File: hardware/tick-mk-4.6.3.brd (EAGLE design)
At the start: 96 x 53 mm, 40 parts, among them IC1 ATMEGA328P, IC2 DS3231, IC3 L7805, Y1 16MHz

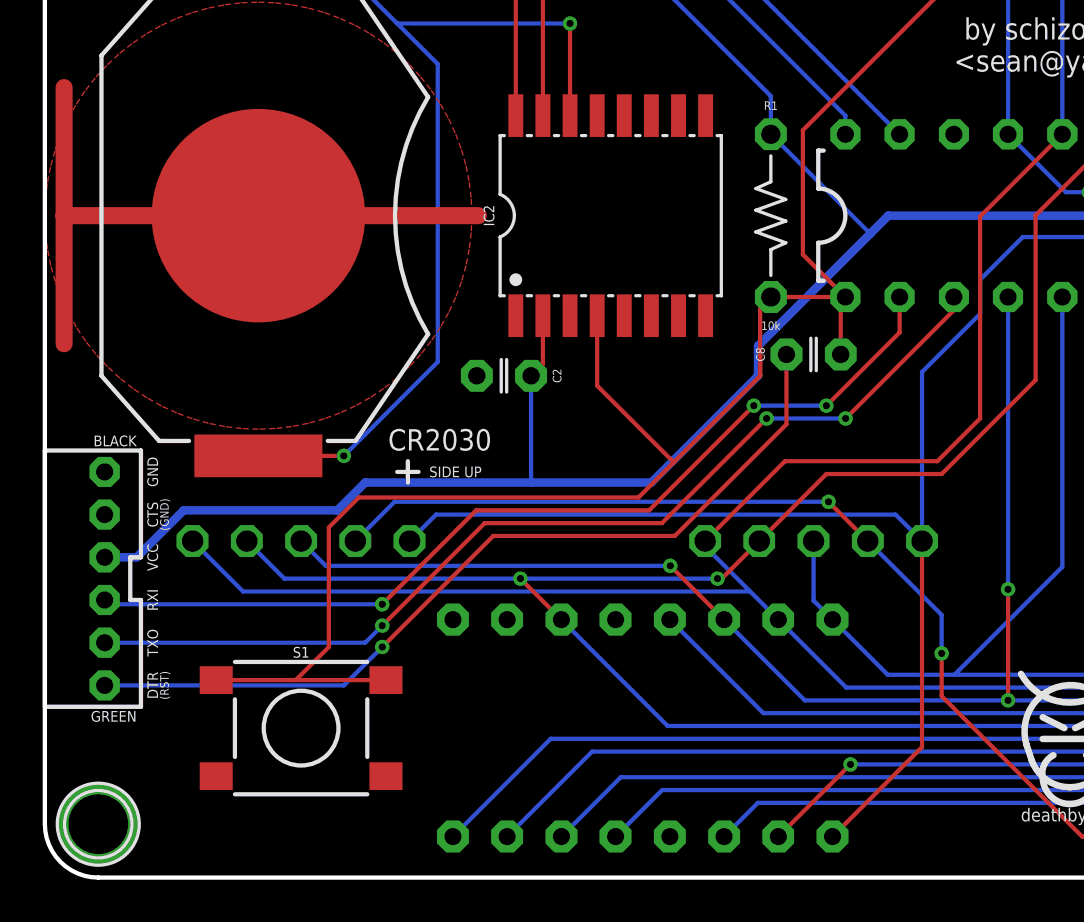
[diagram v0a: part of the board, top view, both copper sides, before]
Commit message: think i'm done fiddling
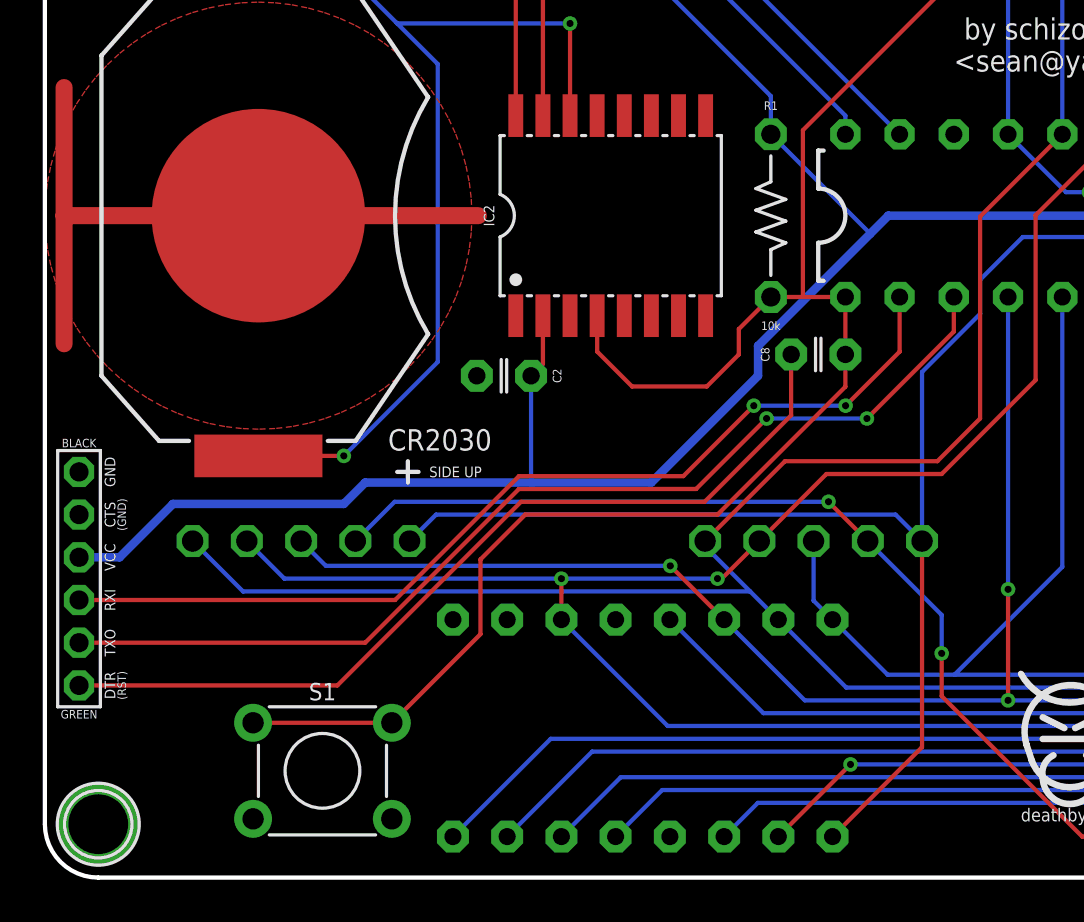
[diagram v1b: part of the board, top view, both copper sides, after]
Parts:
- JP1: value FTDI_CONNJST_PH_VERT_PTH -> FTDI_CONNJST_PH_VERT_PTH_LESSSILK; device A_butts:FTDI_CONN_JST_PH_VERT_PTH -> A_butts:FTDI_CONN_JST_PH_RA_PTH_LESSSILK
- S1: value SPST-NO-TACT6MM-SMD -> SPST-NO-TACT6MM-PTH-SMALL-PADS; device A_butts:DTSM-6 -> A_butts:DTS-6-SMALL-PADS
- moved S1 2.24 mm to (13.0, 5.00)
- moved JP1 1.20 mm to (1.60, 14.0)
- moved C8 0.22 mm to (36.2, 24.5)
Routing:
- net TX: track 46.8 -> 48.6 mm, vias 3 -> 2
- net RX: track 44.2 -> 45.8 mm, vias 3 -> 2
- net RST: track 94.6 -> 93.3 mm
- net VCC: track 149.3 -> 150.5 mm
- net DTR: track 40.3 -> 41.4 mm, vias 1 -> 0
- net A0: track 162.0 -> 161.2 mm
